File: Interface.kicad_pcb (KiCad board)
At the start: 4 copper layers, 126.8 x 95.1 mm, 92 parts, among them J101 AudioJack4, J102 switch, J3 TYPE-C-31-M-12, J4 CONN_DISPLAY, Q1 2N7002VC-7, Q2 2N7002VC-7, U1 W25Q128JVPIQ, U2 RP2040, U3 XC6210B332MR-G, Y1 12MHz

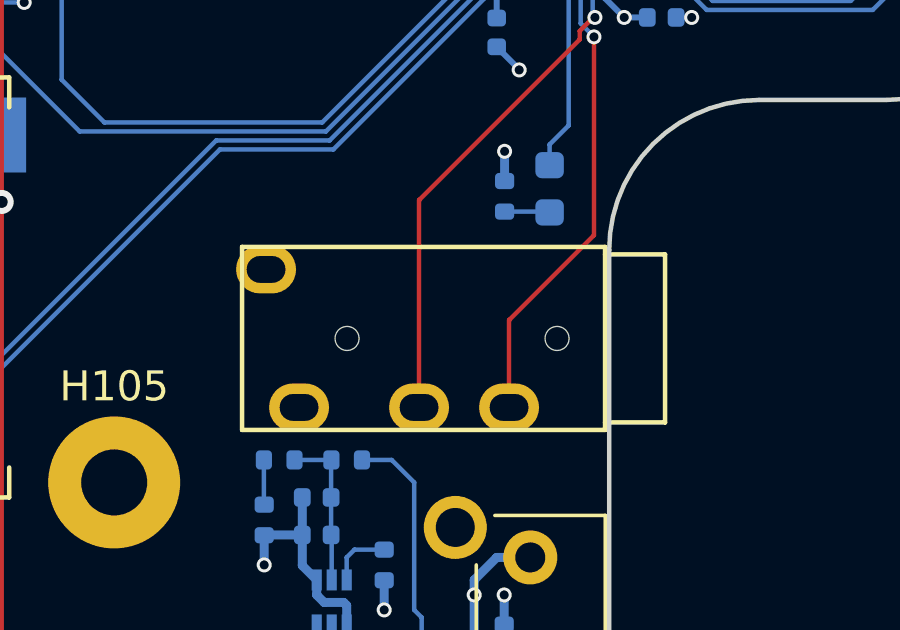
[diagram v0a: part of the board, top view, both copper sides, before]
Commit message: Fix zones
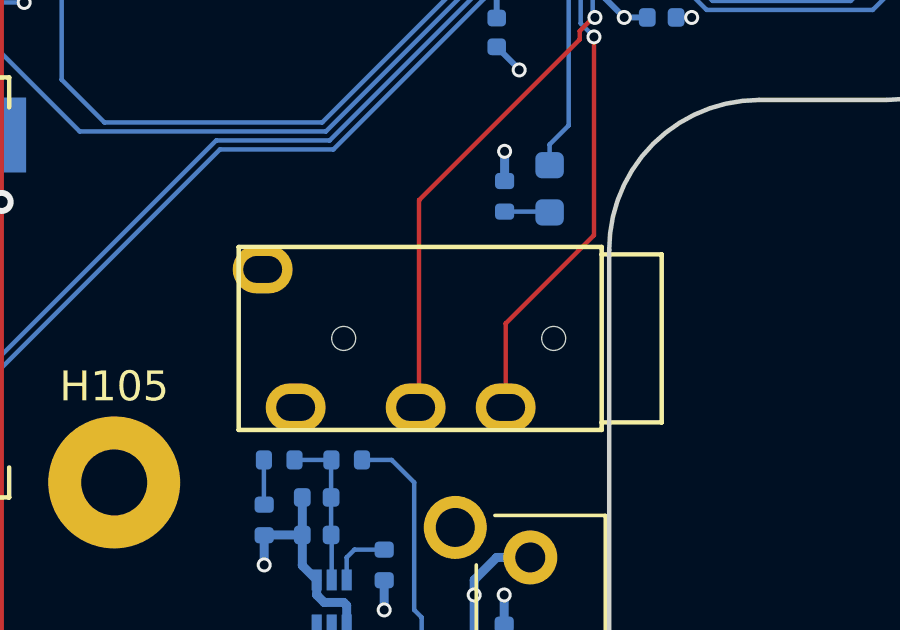
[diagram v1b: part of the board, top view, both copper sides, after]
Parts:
- moved J101 0.11 mm to (134.5, 88.0)
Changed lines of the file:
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@@
     )
     (pad_to_mask_clearance 0)
+    (grid_origin 127.75 43)
     (pcbplotparams
       (layerselection 0x00010fc_ffffffff)
@@
   )
   (footprint "Keyboard:TRRS-PJ-320A" (layer "F.Cu")
-    (at 134.6125 87.95 -90)
+    (at 134.5 87.95 -90)
     (property "Sheetfile" "key-matrix.kicad_sch")
     (property "Sheetname" "Left Matrix")
@@
   (segment (start 135.4375 73.0375) (end 134.5375 73.0375) (width 0.15) (layer "B.Cu") (net 44))
   (segment (start 133.767712 77.701973) (end 133.767712 77.982288) (width 0.15) (layer "F.Cu") (net 45))
-  (segment (start 128.4125 83.3375) (end 128.4125 90.25) (width 0.15) (layer "F.Cu") (net 45))
+  (segment (start 134.2745 77.25) (end 134.219685 77.25) (width 0.15) (layer "F.Cu") (net 45))
+  (segment (start 128.4125 90.1375) (end 128.3 90.25) (width 0.15) (layer "F.Cu") (net 45))
+  (segment (start 128.4125 83.3375) (end 128.4125 90.1375) (width 0.15) (layer "F.Cu") (net 45))
   (segment (start 133.767712 77.982288) (end 128.4125 83.3375) (width 0.15) (layer "F.Cu") (net 45))
   (segment (start 134.219685 77.25) (end 133.767712 77.701973) (width 0.15) (layer "F.Cu") (net 45))
-  (segment (start 134.2745 77.25) (end 134.219685 77.25) (width 0.15) (layer "F.Cu") (net 45))
   (via (at 134.2745 77.25) (size 0.5) (drill 0.3) (layers "F.Cu" "B.Cu") (net 45))
   (segment (start 134.2745 77.25) (end 134.2 77.1755) (width 0.15) (layer "B.Cu") (net 45))
   (segment (start 134.2 77.1755) (end 134.2 75.875) (width 0.15) (layer "B.Cu") (net 45))
+  (segment (start 131.3 87.45) (end 131.3 90.25) (width 0.15) (layer "F.Cu") (net 46))
+  (segment (start 134.242712 84.507288) (end 131.3 87.45) (width 0.15) (layer "F.Cu") (net 46))
   (segment (start 134.242712 77.898725) (end 134.242712 84.507288) (width 0.15) (layer "F.Cu") (net 46))
-  (segment (start 134.242712 84.507288) (end 131.4125 87.3375) (width 0.15) (layer "F.Cu") (net 46))
-  (segment (start 131.4125 87.3375) (end 131.4125 90.25) (width 0.15) (layer "F.Cu") (net 46))
   (via (at 134.242712 77.898725) (size 0.5) (drill 0.3) (layers "F.Cu" "B.Cu") (net 46))
   (segment (start 134.242712 77.892712) (end 133.8 77.45) (width 0.15) (layer "B.Cu") (net 46))
@@
     (polygon
       (pts
-        (xy 139.2 47.5)
-        (xy 139.2 50.9)
+        (xy 128 44.25)
+        (xy 128 46.75)
+        (xy 147.25 46.75)
         (xy 147.3 50.9)
         (xy 147.2 65.8)
@@
         (xy 137.75 78)
         (xy 133.5 82.75)
-        (xy 133.5 102.1)
-        (xy 124.5 102.1)
+        (xy 133.5 102.25)
+        (xy 124.5 102.25)
         (xy 122.25 99.75)
         (xy 122.25 97.25)
-        (xy 122.25 47.75)
+        (xy 122.25 44.25)
       )
     )
@@
     (polygon
       (pts
-        (xy 79.6 37.9)
-        (xy 129.3 38.1)
-        (xy 129.3 45)
-        (xy 139.3 45)
-        (xy 139.3 38.1)
-        (xy 143.5 38.1)
-        (xy 147.7 38.3)
-        (xy 149.1 41.1)
-        (xy 149 75.3)
-        (xy 147 78.3)
-        (xy 140.6 79.6)
-        (xy 136.8 82.2)
-        (xy 134.7 88.1)
-        (xy 134.3 107.4)
-        (xy 125.9 124.9)
-        (xy 122.2 127.6)
-        (xy 118.6 127.7)
-        (xy 102.6 121.9)
-        (xy 78.5 113.5)
-        (xy 59 109.4)
-        (xy 41.5 108.1)
-        (xy 22.4 108)
-        (xy 22.4 50.9)
-        (xy 41.5 50.9)
-        (xy 41.5 37.9)
-        (xy 60.5 37.9)
-        (xy 60.5 31.9)
-        (xy 79.6 31.9)
+        (xy 124.5 102.25)
+        (xy 122.25 99.75)
+        (xy 122.25 75.5)
+        (xy 119.75 75.5)
+        (xy 119.75 70.25)
+        (xy 122.25 70.25)
+        (xy 122.25 44.25)
+        (xy 126.25 44.25)
+        (xy 126.25 43)
+        (xy 127.25 43)
+        (xy 127.25 44.25)
+        (xy 128 44.25)
+        (xy 128 46.75)
+        (xy 129.75 46.75)
+        (xy 129.75 46)
+        (xy 130.75 46)
+        (xy 130.75 46.75)
+        (xy 138.25 46.75)
+        (xy 138.25 46)
+        (xy 139.244231 46)
+        (xy 139.25 46.75)
+        (xy 141 46.75)
+        (xy 141 44.25)
+        (xy 147.25 44.25)
+        (xy 147 78)
+        (xy 137.75 78)
+        (xy 133.5 82.75)
+        (xy 133.5 102.25)
       )
     )
